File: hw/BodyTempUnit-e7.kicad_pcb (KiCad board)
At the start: 4 copper layers, 25 x 30 mm, 27 parts, among them IC1 MAX481CUA, IC2 MEGA8-MI, U1 MAX30205MTA+21-0137I_T833-2-M, U2 LSM6DS3, U3 MCP1801T-3302I_OT

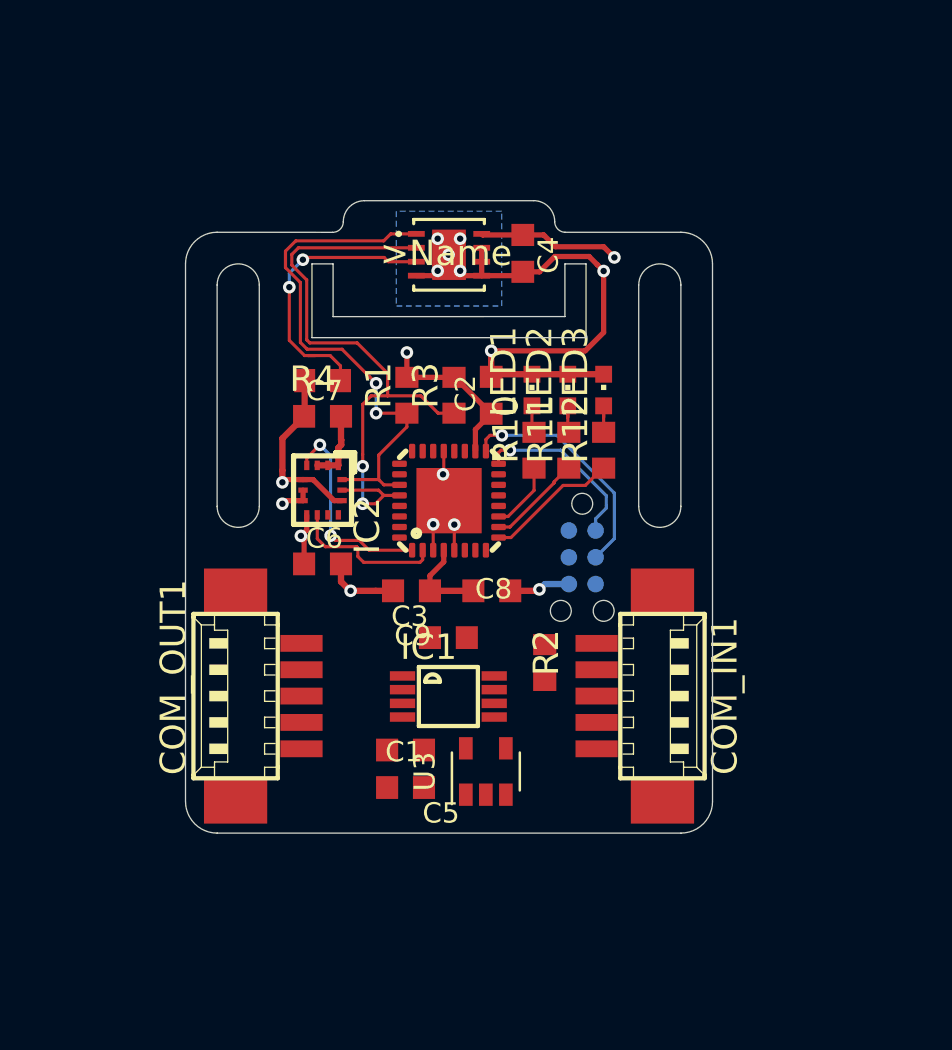
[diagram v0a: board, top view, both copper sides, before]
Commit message: some rerouting
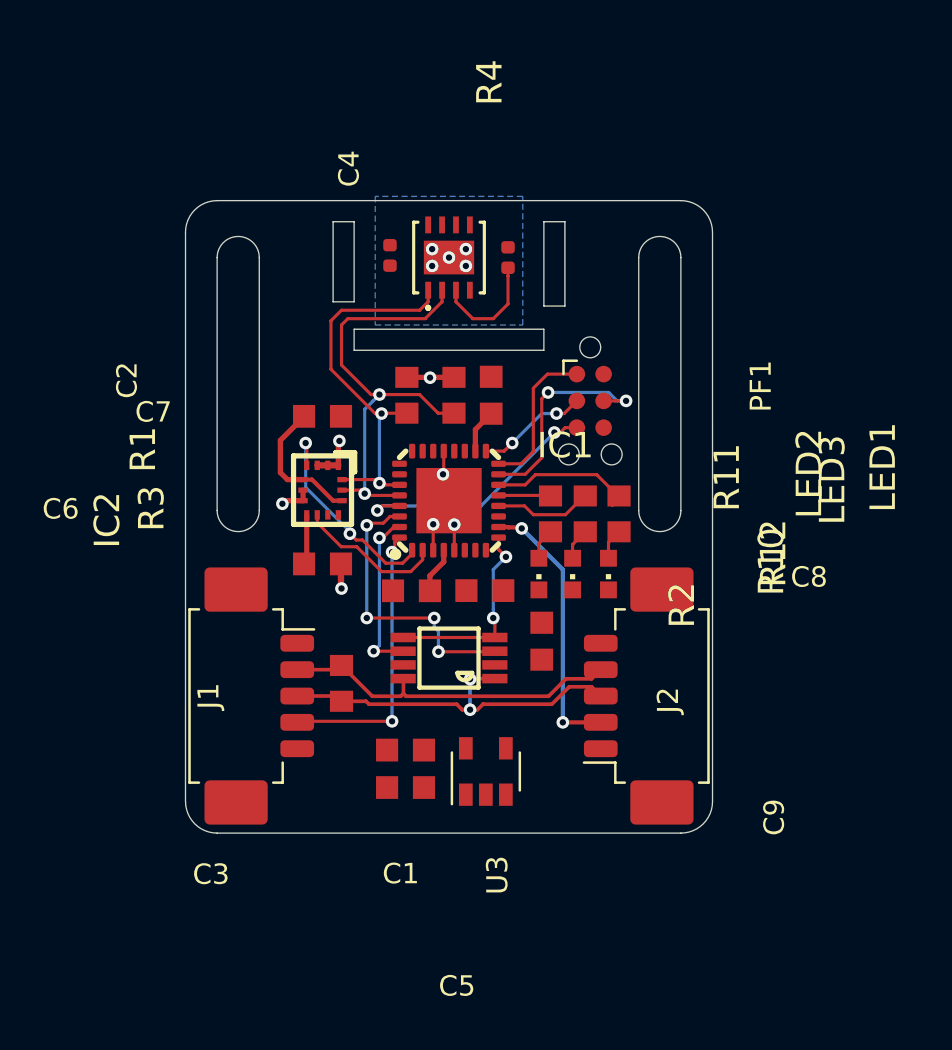
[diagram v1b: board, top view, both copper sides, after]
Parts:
- removed COM_IN1, COM_OUT1: 53?-05261, BodyTempUnit-e7:53261-05
- added J1: CONN_IN, Connector_Molex:Molex_PicoBlade_53261-0571_1x05-1MP_P1.25mm_Horizontal, F.Cu at (67.9, 128.5)
- added J2: CONN_OUT, Connector_Molex:Molex_PicoBlade_53261-0571_1x05-1MP_P1.25mm_Horizontal, F.Cu at (87.1, 128.5)
- C4: footprint BodyTempUnit-e7:C0603K -> Capacitor_SMD:C_0402_1005Metric
- PF1: moved to F.Cu
- R4: footprint BodyTempUnit-e7:R0603 -> Resistor_SMD:R_0402_1005Metric
- moved R4 10.6 mm to (80.3, 107.7), turned to 90 degrees
- moved R2 9.69 mm to (72.4, 127.9)
- moved LED1 9.45 mm to (85.1, 122.7), turned to 180 degrees
- moved LED3 8.85 mm to (83.4, 122.7), turned to 180 degrees
- moved LED2 8.84 mm to (81.8, 122.7), turned to 180 degrees
- moved PF1 7.43 mm to (84.2, 114.5)
- moved C4 6.30 mm to (74.7, 107.6)
- moved R10 5.04 mm to (85.6, 119.9), turned to 270 degrees
- moved C9 4.43 mm to (81.9, 125.9), turned to 90 degrees
- moved R12 3.14 mm to (84.0, 119.9), turned to 270 degrees
- moved R11 3.14 mm to (82.3, 119.9), turned to 270 degrees
- moved IC1 1.82 mm to (77.5, 126.7), turned to 90 degrees
- moved C8 0.33 mm to (79.2, 123.5)
- moved U1 0.13 mm to (77.5, 107.7), turned to 90 degrees
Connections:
- IC2 pad 10: Net-(IC2-Pad10) -> /SIG_OUT
- IC2 pad 12: /SIG_OUT -> Net-(IC2-Pad12)
- R12 pad 1: Net-(IC2-Pad11) -> Net-(IC2-Pad12)
- U1 pad 5: GND -> VCC
- U1 pad 6: GND -> VCC
- U1 pad 7: GND -> VCC
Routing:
- net GND: track 44.9 -> 12.6 mm, vias 13 -> 11
- net /RS485_-: track 0.00 -> 18.0 mm, vias 0 -> 2
- net /RS485_+: track 0.00 -> 16.4 mm
- net VCC: track 30.1 -> 15.6 mm, vias 4 -> 1
- net /RS485_RO: track 0.00 -> 13.7 mm, vias 0 -> 4
- net /SIG_IN: track 0.25 -> 13.7 mm, vias 0 -> 2
- net /SIG_OUT: track 0.00 -> 12.9 mm, vias 0 -> 2
- net /RST: track 0.00 -> 12.2 mm, vias 0 -> 2
- net /MOSI: track 0.00 -> 10.2 mm, vias 0 -> 2
- net /RS485_DE: track 0.00 -> 9.52 mm, vias 0 -> 2
- net /U1_OS: track 13.6 -> 5.36 mm, vias 2 -> 0
- net /RS485_DI: track 0.00 -> 8.05 mm, vias 0 -> 2
- net /SCL: track 29.5 -> 21.8 mm
- net /SDA: track 25.0 -> 18.6 mm
- net Net-(IC2-Pad11): track 6.35 -> 0.00 mm
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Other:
- outline, holes or cut-outs redrawn
- net class Default: trace_width 0.25 -> 0.2
- rule via_min_drill: 0.3 -> 0.2
- rule via_min_size: 0.4 -> 0.45
